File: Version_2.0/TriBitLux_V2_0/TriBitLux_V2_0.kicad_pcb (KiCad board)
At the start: 2 copper layers, 87.7 x 45.4 mm, 38 parts, among them J2 Conn_01x02_Pin, U1 LM339, U2 LM339, U3 74LS148, U4 74LS48, U5 D198K

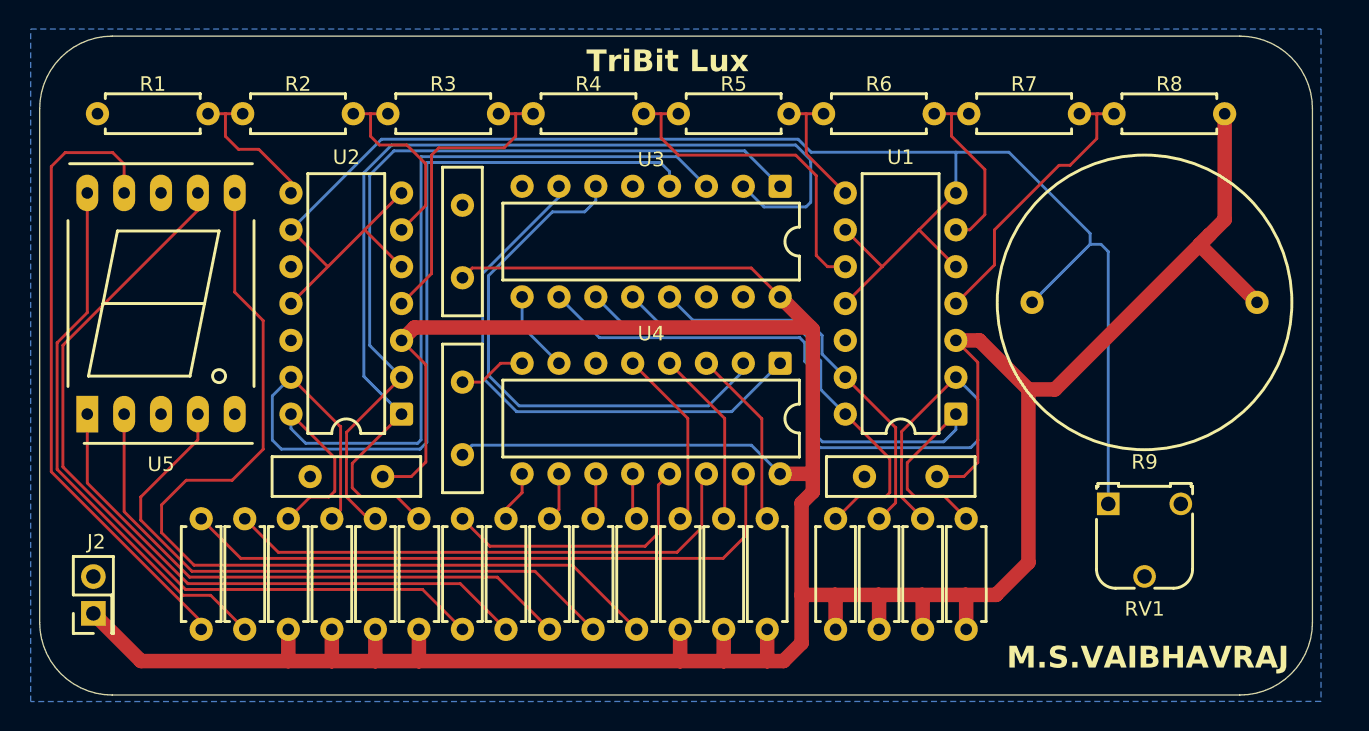
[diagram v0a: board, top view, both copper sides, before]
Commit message: 3V3 Design Update
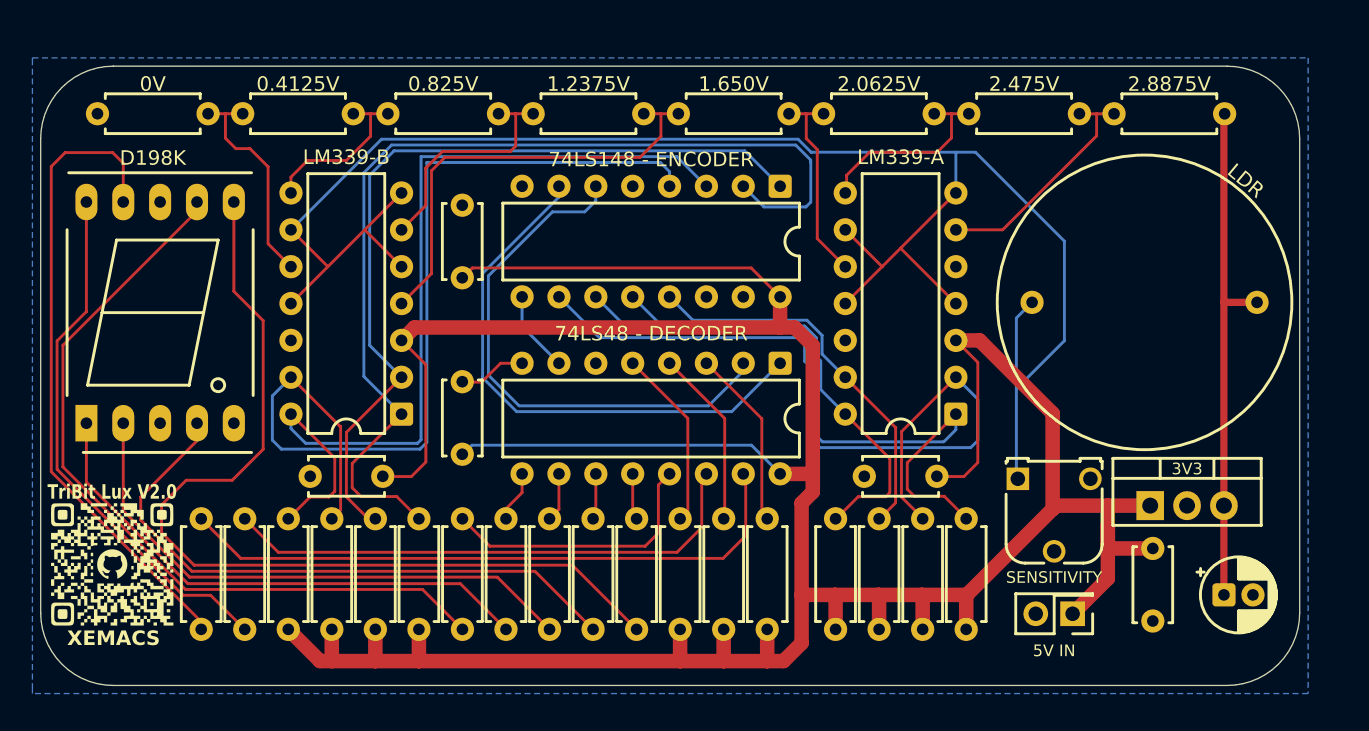
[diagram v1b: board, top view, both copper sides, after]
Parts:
- added C5: 0.1u, Extra Footprints:C_Disc_D5.0mm_W2.5mm_P5.00mm_ClearSilk, F.Cu at (197.9, 124.8)
- added C6: 2.2u, Extra Footprints:CP_Radial_D5.0mm_P2.00mm_ClearSilk, F.Cu at (202.8, 128.0)
- added G***: LOGO, Extra Footprints:QR, F.Cu at (126.2, 125.9)
- added U6: SPX2920U-3.3_TO220, Package_TO_SOT_THT:TO-220-3_Vertical, F.Cu at (197.7, 121.8)
- C1, C2, C3, C4: footprint Capacitor_THT:C_Disc_D10.0mm_W2.5mm_P5.00mm -> Extra Footprints:C_Disc_D5.0mm_W2.5mm_P5.00mm_ClearSilk
- RV1: value R_Potentiometer -> 10k
- moved J2 67.5 mm to (192.4, 129.3), turned to 180 degrees
- moved RV1 6.47 mm to (188.6, 120.0)
- moved U5 0.63 mm to (124.4, 116.2)
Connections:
- R1 pad 1: VDD -> /3.3V
- R1 pad 2: Net-(U1A--) -> /2.8875V
- R2 pad 1: Net-(U1A--) -> /2.8875V
- R2 pad 2: Net-(U1B--) -> /2.475V
- R3 pad 1: Net-(U1B--) -> /2.475V
- R3 pad 2: Net-(U1D--) -> /2.0625V
- R4 pad 1: Net-(U1D--) -> /2.0625V
- R4 pad 2: Net-(U1C--) -> /1.650V
- R5 pad 1: Net-(U1C--) -> /1.650V
- R5 pad 2: Net-(U2A--) -> /1.2375V
- R6 pad 1: Net-(U2A--) -> /1.2375V
- R6 pad 2: Net-(U2B--) -> /0.825V
- R7 pad 1: Net-(U2B--) -> /0.825V
- R7 pad 2: Net-(U2D--) -> /0.4125V
- R8 pad 1: Net-(U2D--) -> /0.4125V
- R9 pad 1: Net-(U1A-+) -> /Input Voltage
- R9 pad 2: VDD -> /3.3V
- RV1 pad 1: Net-(U1A-+) -> /Input Voltage
- U1 pad 10: Net-(U1C--) -> /2.0625V
- U1 pad 11: Net-(U1A-+) -> /Input Voltage
- U1 pad 4: Net-(U1A--) -> /Input Voltage
- U1 pad 5: Net-(U1A-+) -> GND
- U1 pad 6: Net-(U1B--) -> /2.8875V
- U1 pad 7: Net-(U1A-+) -> /Input Voltage
- U1 pad 8: Net-(U1D--) -> /2.475V
- U1 pad 9: Net-(U1A-+) -> /Input Voltage
- U2 pad 10: GND -> /0.4125V
- U2 pad 11: Net-(U1A-+) -> /Input Voltage
- U2 pad 4: Net-(U2A--) -> /1.650V
- U2 pad 5: Net-(U1A-+) -> /Input Voltage
- U2 pad 6: Net-(U2B--) -> /1.2375V
- U2 pad 7: Net-(U1A-+) -> /Input Voltage
- U2 pad 8: Net-(U2D--) -> /0.825V
- U2 pad 9: Net-(U1A-+) -> /Input Voltage
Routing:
- net Net-(U1A-+): track 124.4 -> 0.00 mm
- net /Input Voltage: track 0.00 -> 123.6 mm
- net /3.3V: track 0.00 -> 36.0 mm
- net /1.650V: track 0.00 -> 30.8 mm
- net VDD: track 269.4 -> 239.7 mm
- net Net-(U1C--): track 23.7 -> 0.00 mm
- net Net-(U2A--): track 21.4 -> 0.00 mm
- net Net-(U1A--): track 20.0 -> 0.00 mm
- net /1.2375V: track 0.00 -> 16.4 mm
- net /2.8875V: track 0.00 -> 16.3 mm
- net /0.4125V: track 0.00 -> 15.4 mm
- net /2.0625V: track 0.00 -> 14.0 mm
- net Net-(U2B--): track 13.8 -> 0.00 mm
- net /2.475V: track 0.00 -> 13.6 mm
- net Net-(U1B--): track 12.7 -> 0.00 mm
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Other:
- board size 87.7 x 45.4 mm -> 86.8 x 42.7 mm
- board text added: "0.4125V"
- board text added: "0.825V"
- board text added: "0V"
- board text added: "1.2375V"
- board text added: "1.650V"
- board text added: "2.0625V"
- board text added: "2.475V"
- board text added: "2.8875V"
- board text added: "3V3"
- board text added: "5V IN"
- board text added: "74LS148 - ENCODER"
- board text added: "74LS48 - DECODER"
- board text added: "D198K"
- board text added: "LDR"
- board text added: "LM339-A"
- board text added: "LM339-B"
- board text added: "SENSITIVITY"
- board text added: "TriBit Lux V2.0"
- board text added: "XEMACS"
- board text removed: "M.S.VAIBHAVRAJ"
- board text removed: "TriBit Lux"
